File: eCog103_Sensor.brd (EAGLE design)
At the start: 48 x 28 mm, 7 parts

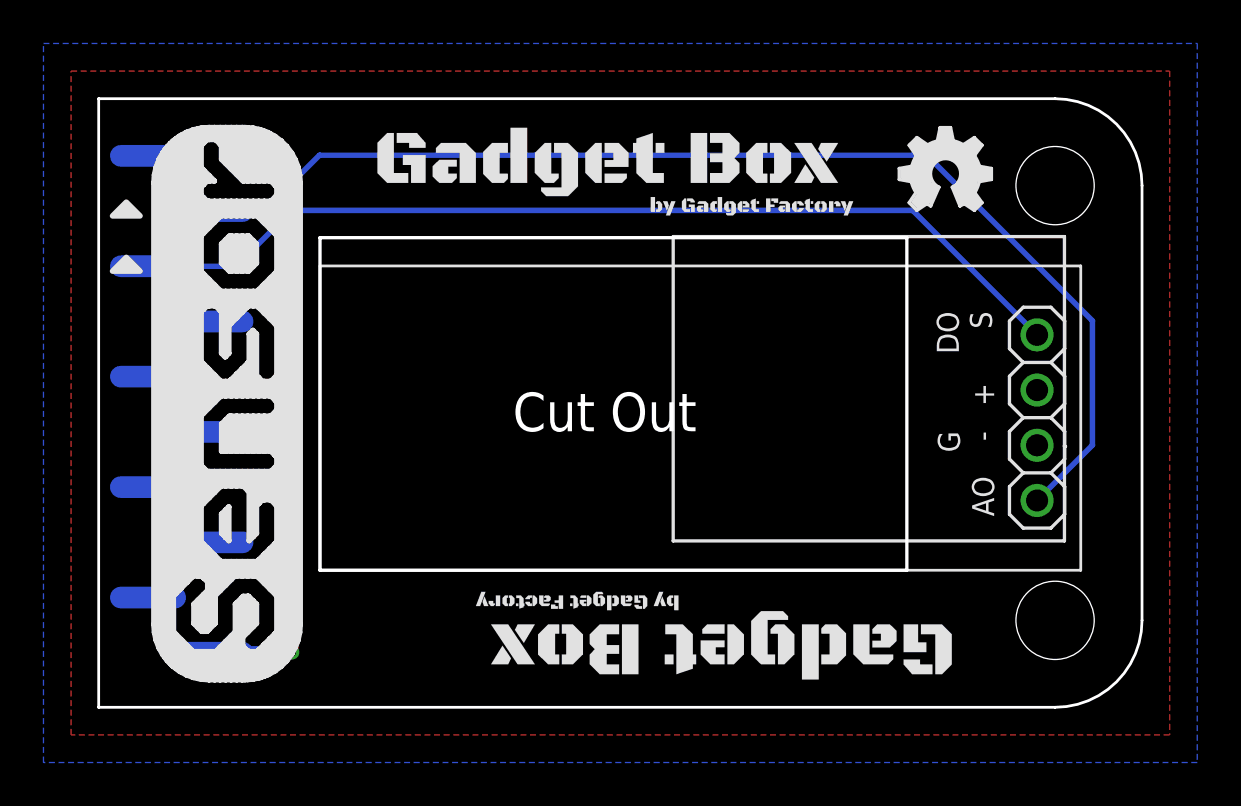
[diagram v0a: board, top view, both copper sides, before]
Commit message: All the 2.0 updates
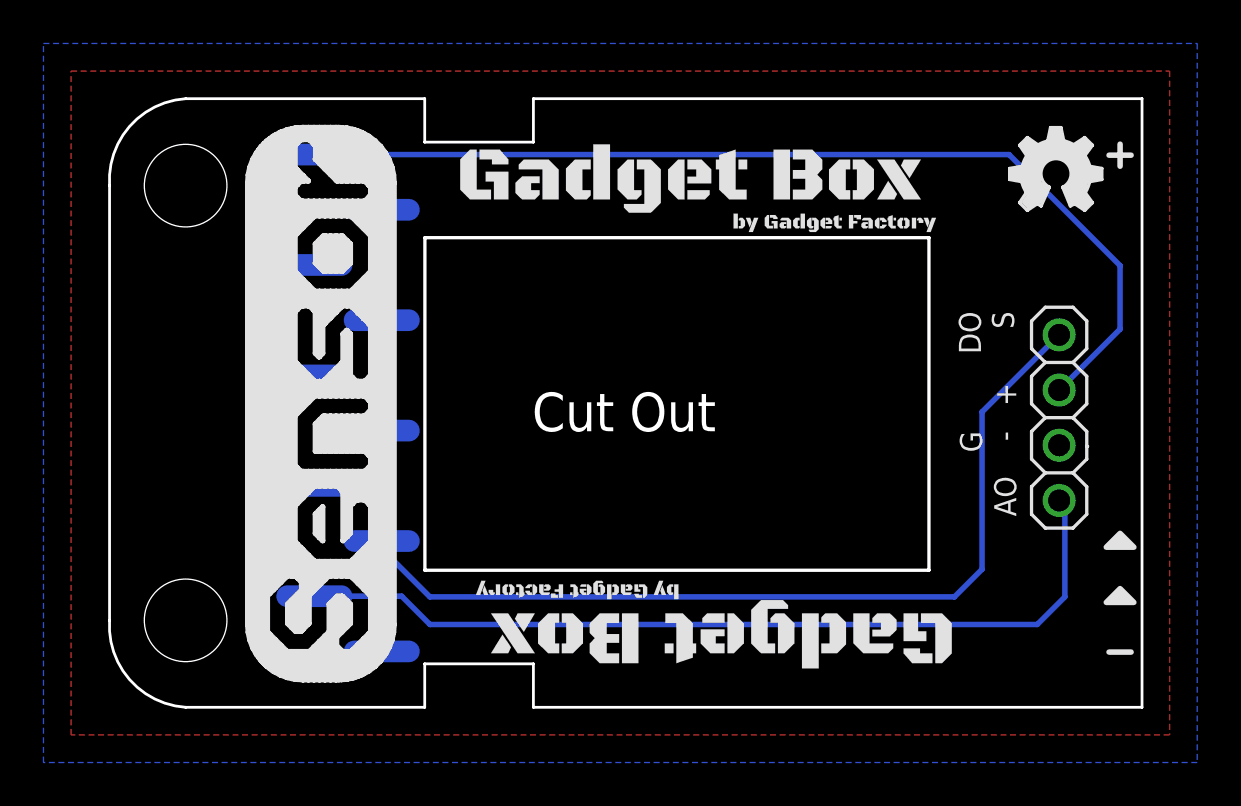
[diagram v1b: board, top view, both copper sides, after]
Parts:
- moved U$2 48.2 mm to (47.0, 7.62)
- moved U$3 48.2 mm to (47.0, 5.08)
- moved U$5 5.08 mm to (41.9, 22.9)
- moved U$4 3.89 mm to (27.3, 24.3)
- moved U$1 1.02 mm to (46.2, 13.3)
- moved U$6 0.51 mm to (28.6, 3.43)
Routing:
- net 3V3: track 4.80 -> 46.1 mm, vias 1 -> 0
- net A1: track 53.9 -> 40.1 mm
- net A2: track 44.3 -> 41.7 mm
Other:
- board size 48 x 28 mm -> 47.5 x 28 mm
- board text added: "0"
- board text added: "1"
- board text added: "ecog103 v2.0"
- board text removed: "ecog103 v1.2"
